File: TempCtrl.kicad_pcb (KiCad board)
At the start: 2 copper layers, 23 parts, among them P1 PWR 18V, P2 CONN_01X05, Q1 BD678, U1 LM358

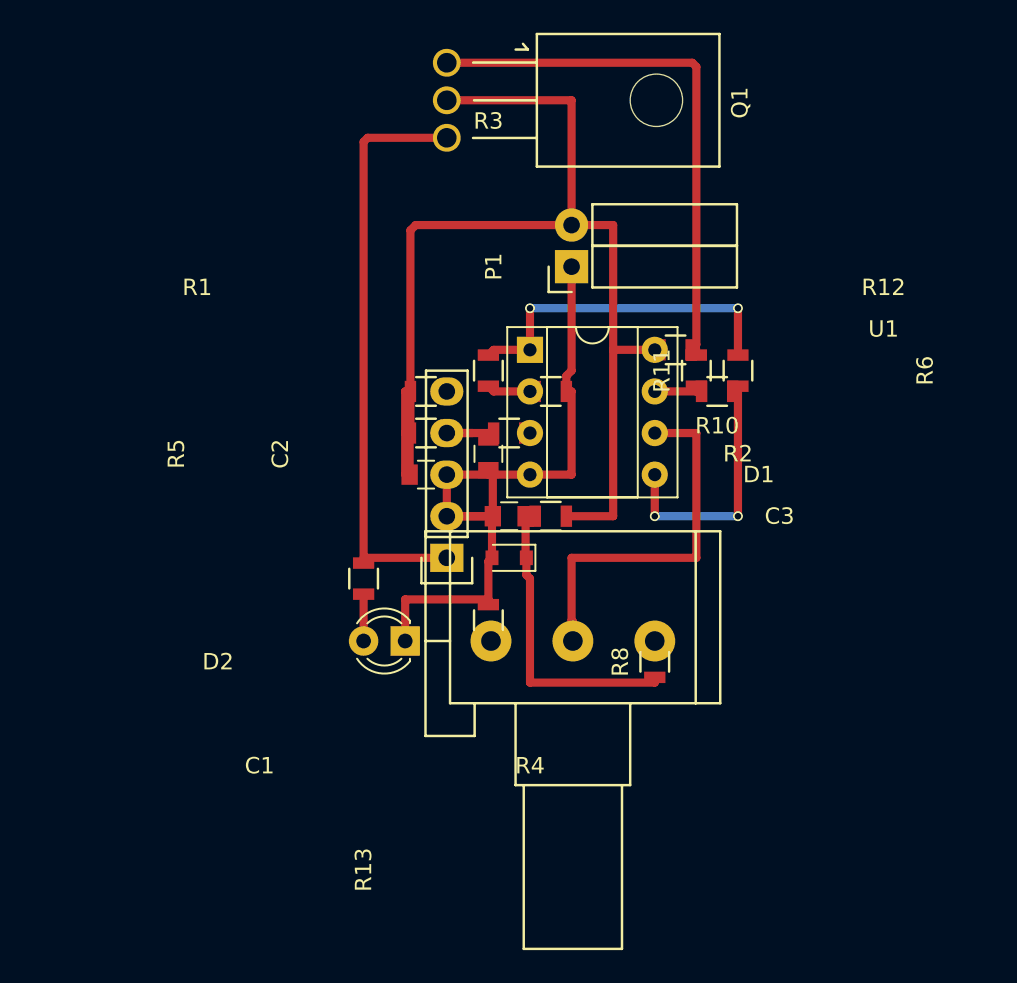
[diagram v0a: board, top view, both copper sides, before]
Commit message: Added PNG images
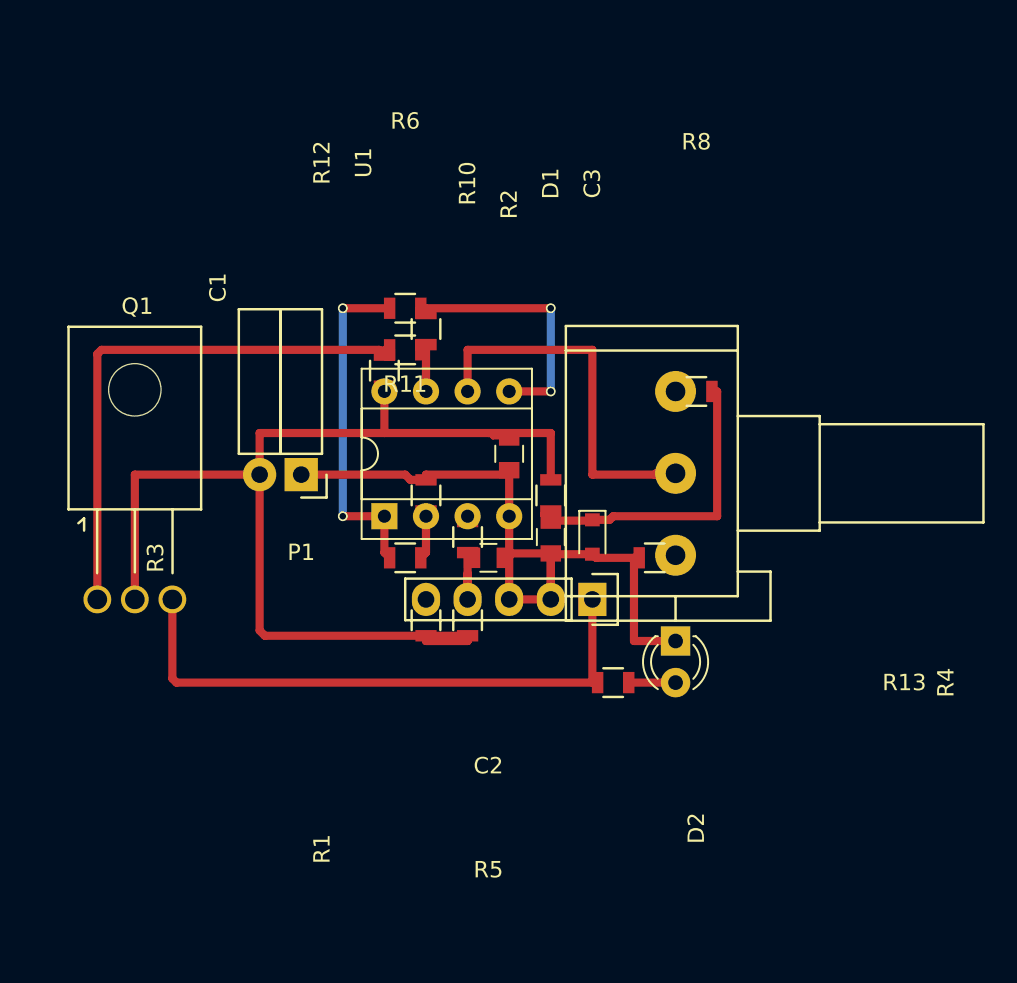
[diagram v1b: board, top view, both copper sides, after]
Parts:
- moved Q1 35.9 mm to (156.2, 106.7), turned to 0 degrees
- moved P1 20.8 mm to (166.4, 99.1), turned to 180 degrees
- moved R6 20.7 mm to (172.7, 88.9), turned to 180 degrees
- moved R10 18.2 mm to (174.0, 90.2), turned to 270 degrees
- moved R11 17.8 mm to (172.7, 91.4), turned to 180 degrees
- moved R12 17.8 mm to (171.4, 92.7), turned to 270 degrees
- moved R8 16.7 mm to (190.5, 94.0), turned to 180 degrees
- moved D2 16.5 mm to (189.2, 109.2), turned to 270 degrees
- moved R13 16.5 mm to (185.4, 111.8), turned to 180 degrees
- moved RV1 15.3 mm to (189.2, 94.0), turned to 0 degrees
- moved R1 14.0 mm to (174.0, 108.0), turned to 90 degrees
- moved U1 13.5 mm to (171.4, 101.6), turned to 90 degrees
- moved R5 12.5 mm to (172.7, 104.1), turned to 180 degrees
- moved R2 11.7 mm to (176.5, 108.0), turned to 90 degrees
- moved R9 10.9 mm to (188.0, 104.1), turned to 180 degrees
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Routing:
- net VCC: track 73.4 -> 69.4 mm

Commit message: Final version
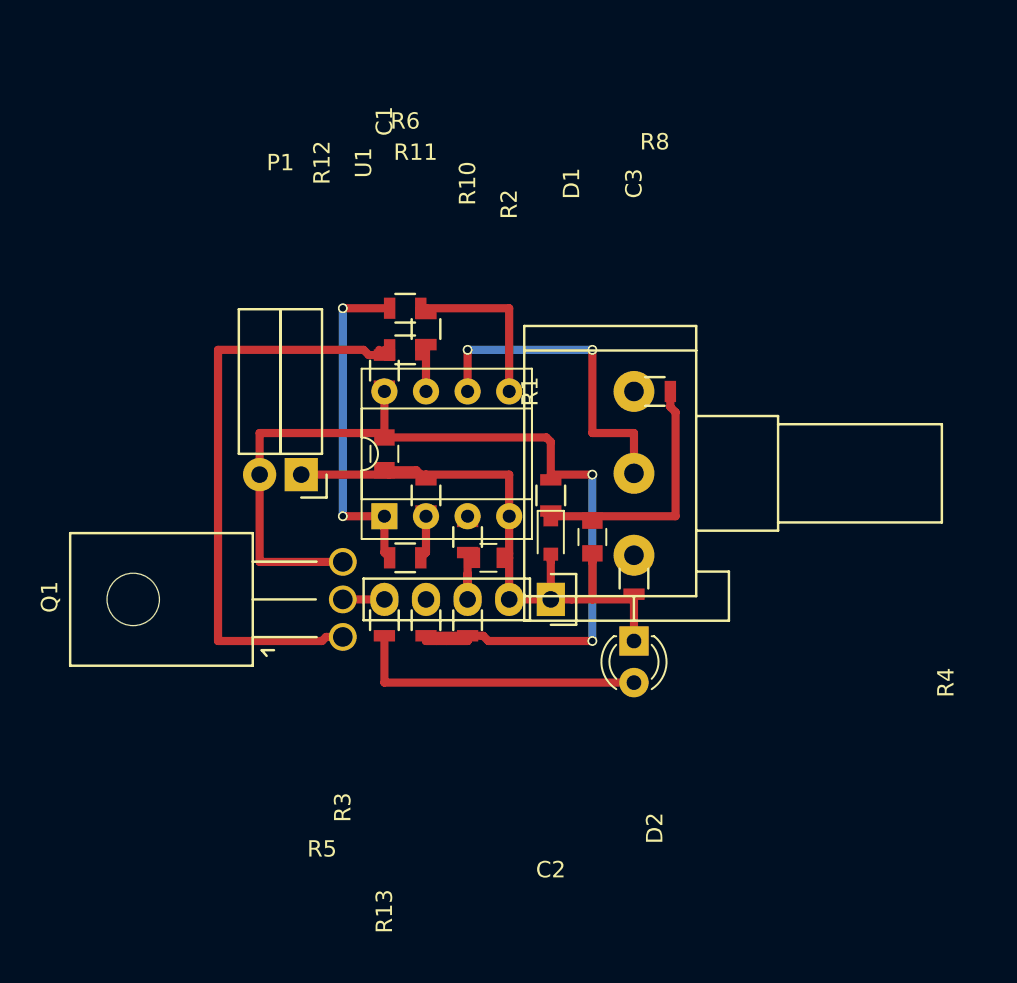
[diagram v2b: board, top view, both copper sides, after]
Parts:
- P1: value PWR 18V -> PWR 18-24V
- moved R13 14.5 mm to (171.4, 108.0), turned to 90 degrees
- moved Q1 12.7 mm to (168.9, 106.7), turned to 90 degrees
- moved C1 7.62 mm to (171.4, 97.8)
- moved C3 2.54 mm to (184.2, 102.9)
- moved D1 2.54 mm to (181.6, 102.9)
- moved D2 2.54 mm to (186.7, 109.2)
- moved P2 2.54 mm to (181.6, 106.7)
- moved R8 2.54 mm to (188.0, 94.0)
- moved RV1 2.54 mm to (186.7, 94.0)
- moved R9 1.80 mm to (186.7, 105.4), turned to 270 degrees
- turned R1 to 270 degrees
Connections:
- P2 pad 1: Net-(P2-Pad1) -> GNDREF
- P2 pad 3: GNDREF -> Net-(C2-Pad1)
- P2 pad 4: Net-(C2-Pad1) -> Net-(P2-Pad4)
- Q1 pad 2: VCC -> Net-(P2-Pad5)
- Q1 pad 3: Net-(P2-Pad1) -> VCC
- R1 pad 1: VCC -> Net-(P2-Pad4)
- R1 pad 2: Net-(P2-Pad5) -> VCC
- R13 pad 2: Net-(P2-Pad1) -> Net-(P2-Pad5)
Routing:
- net Net-(P2-Pad1): track 36.0 -> 0.00 mm
- net Net-(D2-Pad2): track 2.86 -> 18.1 mm
- net VCC: track 69.4 -> 63.8 mm, vias 0 -> 2
- net Net-(R10-Pad1): track 15.6 -> 10.8 mm, vias 2 -> 0
- net Net-(Q1-Pad1): track 33.1 -> 37.0 mm
- net GNDREF: track 45.0 -> 41.8 mm
- net Net-(RV1-Pad2): track 22.9 -> 20.2 mm, vias 0 -> 2
- net Net-(P2-Pad5): track 0.00 -> 2.54 mm
- net Net-(C3-Pad2): track 18.2 -> 16.0 mm
